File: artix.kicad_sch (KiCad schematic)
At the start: 50 parts, among them U2 XC7A200T-FBG484

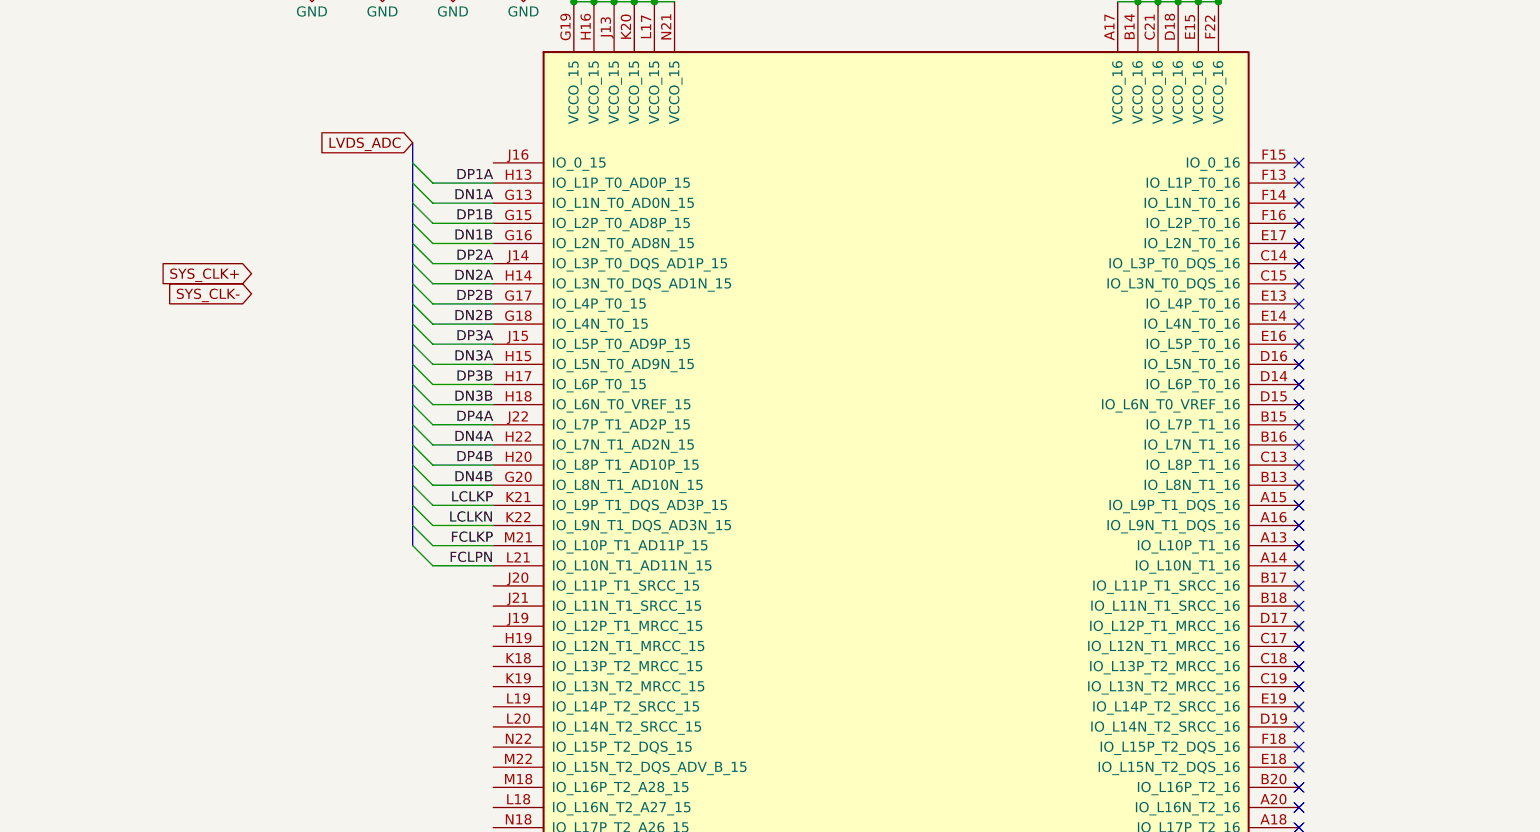
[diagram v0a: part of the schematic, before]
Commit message: added clk
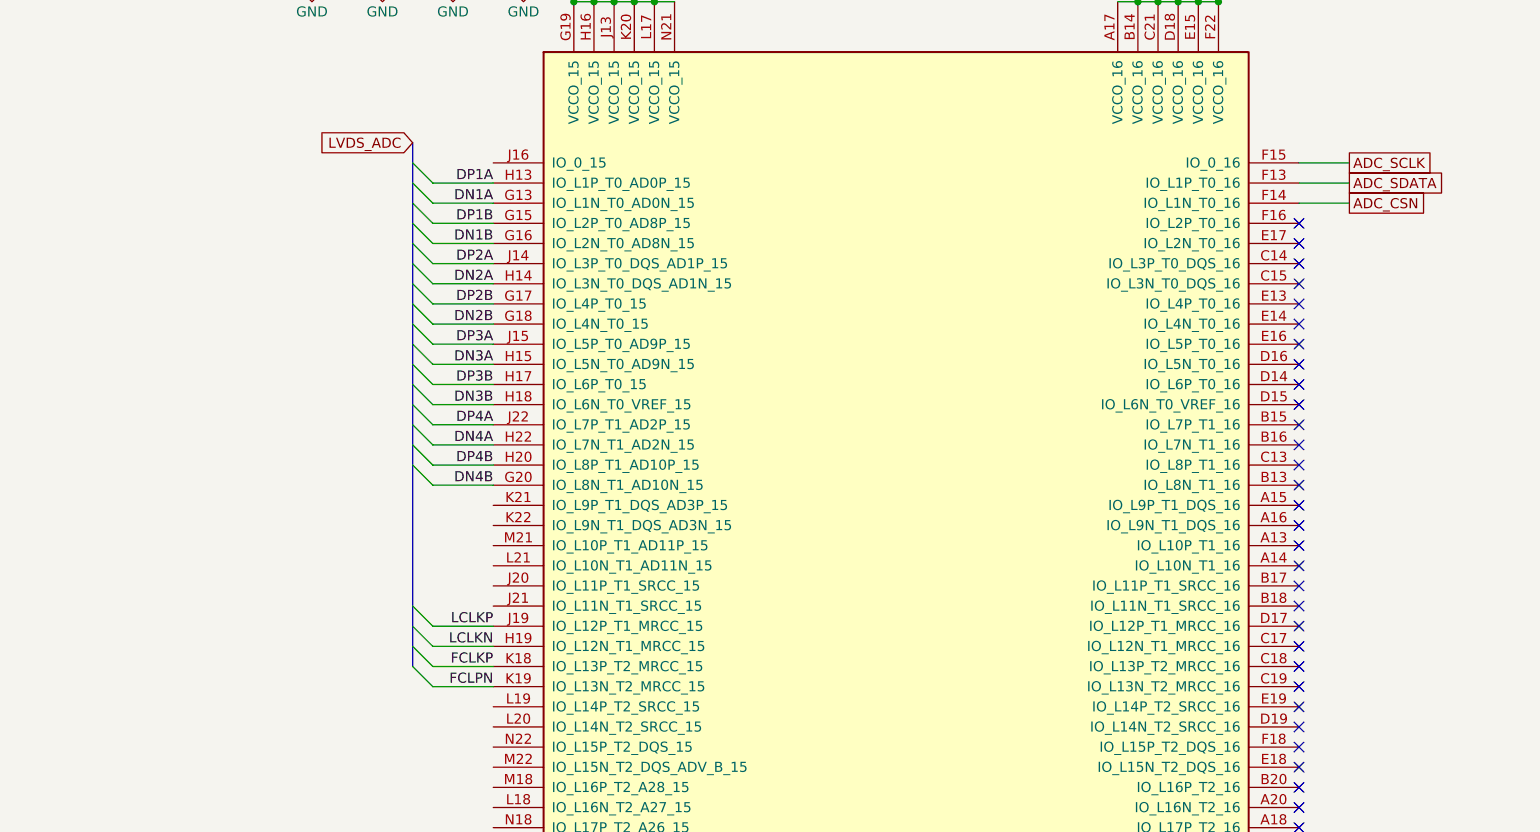
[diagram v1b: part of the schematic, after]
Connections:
- net FCLKP: now also U2.K18 (IO_L13P_T2_MRCC_15); no longer U2.M21 (IO_L10P_T1_AD11P_15)
- net FCLPN: now also U2.K19 (IO_L13N_T2_MRCC_15); no longer U2.L21 (IO_L10N_T1_AD11N_15)
- net LCLKN: now also U2.H19 (IO_L12N_T1_MRCC_15); no longer U2.K22 (IO_L9N_T1_DQS_AD3N_15)
- net LCLKP: now also U2.J19 (IO_L12P_T1_MRCC_15); no longer U2.K21 (IO_L9P_T1_DQS_AD3P_15)
- net ADC_SDATA: now reaches U2.F13 (IO_L1P_T0_16)
- net ADC_CSN: now reaches U2.F14 (IO_L1N_T0_16)
- net ADC_SCLK: now reaches U2.F15 (IO_0_16)
- no-connect marks 180 -> 177
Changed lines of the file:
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@@
 	)
 	(no_connect
-		(at 541.02 92.71)
-	)
-	(no_connect
 		(at 541.02 143.51)
 	)
 	(no_connect
-		(at 541.02 97.79)
-	)
-	(no_connect
 		(at 541.02 207.01)
 	)
@@
 	)
 	(no_connect
-		(at 541.02 95.25)
-	)
-	(no_connect
 		(at 140.97 176.53)
 	)
@@
 	)
 	(bus_entry
-		(at 431.8 95.25)
+		(at 431.8 158.75)
 		(size -2.54 -2.54)
 		(stroke
@@
 	)
 	(bus_entry
-		(at 431.8 135.89)
+		(at 431.8 95.25)
 		(size -2.54 -2.54)
 		(stroke
@@
 	)
 	(bus_entry
-		(at 431.8 110.49)
+		(at 431.8 153.67)
 		(size -2.54 -2.54)
 		(stroke
@@
 	)
 	(bus_entry
-		(at 431.8 128.27)
+		(at 431.8 110.49)
 		(size -2.54 -2.54)
 		(stroke
@@
 	)
 	(bus_entry
-		(at 431.8 140.97)
+		(at 431.8 128.27)
 		(size -2.54 -2.54)
 		(stroke
@@
 	)
 	(bus_entry
-		(at 431.8 143.51)
+		(at 431.8 151.13)
 		(size -2.54 -2.54)
 		(stroke
@@
 	)
 	(bus_entry
-		(at 431.8 138.43)
+		(at 431.8 105.41)
 		(size -2.54 -2.54)
 		(stroke
@@
 	)
 	(bus_entry
-		(at 431.8 105.41)
+		(at 431.8 156.21)
 		(size -2.54 -2.54)
 		(stroke
@@
 	(wire
 		(pts
-			(xy 439.42 138.43) (xy 431.8 138.43)
+			(xy 238.76 49.53) (xy 238.76 50.8)
 		)
 		(stroke
@@
 	(wire
 		(pts
-			(xy 238.76 49.53) (xy 238.76 50.8)
+			(xy 22.86 41.91) (xy 22.86 43.18)
 		)
 		(stroke
@@
 	(wire
 		(pts
-			(xy 22.86 41.91) (xy 22.86 43.18)
+			(xy 439.42 158.75) (xy 431.8 158.75)
 		)
 		(stroke
@@
 	(wire
 		(pts
+			(xy 541.02 97.79) (xy 547.37 97.79)
+		)
+		(stroke
+			(width 0)
+			(type default)
+		)
+	)
+	(wire
+		(pts
 			(xy 380.365 60.96) (xy 380.365 61.595)
 		)
@@
 	(wire
 		(pts
-			(xy 439.42 135.89) (xy 431.8 135.89)
+			(xy 273.05 293.37) (xy 284.48 293.37)
 		)
 		(stroke
@@
 	(wire
 		(pts
-			(xy 273.05 293.37) (xy 284.48 293.37)
+			(xy 541.02 95.25) (xy 547.37 95.25)
 		)
 		(stroke
@@
 	(bus
 		(pts
-			(xy 429.26 90.17) (xy 429.26 140.97)
+			(xy 429.26 90.17) (xy 429.26 156.21)
 		)
 		(stroke
@@
 	(wire
 		(pts
-			(xy 439.42 143.51) (xy 431.8 143.51)
+			(xy 541.02 92.71) (xy 547.37 92.71)
 		)
 		(stroke
@@
 	(wire
 		(pts
+			(xy 439.42 153.67) (xy 431.8 153.67)
+		)
+		(stroke
+			(width 0)
+			(type default)
+		)
+	)
+	(wire
+		(pts
 			(xy 439.42 105.41) (xy 431.8 105.41)
 		)
@@
 	(wire
 		(pts
+			(xy 439.42 156.21) (xy 431.8 156.21)
+		)
+		(stroke
+			(width 0)
+			(type default)
+		)
+	)
+	(wire
+		(pts
 			(xy 425.45 55.88) (xy 425.45 57.15)
 		)
@@
 	(wire
 		(pts
-			(xy 439.42 140.97) (xy 431.8 140.97)
-		)
-		(stroke
-			(width 0)
-			(type default)
-		)
-	)
-	(wire
-		(pts
 			(xy 146.05 48.26) (xy 146.05 48.895)
 		)
@@
 	(wire
 		(pts
+			(xy 439.42 151.13) (xy 431.8 151.13)
+		)
+		(stroke
+			(width 0)
+			(type default)
+		)
+	)
+	(wire
+		(pts
 			(xy 546.1 50.8) (xy 546.1 52.07)
 		)
@@
 		)
 	)
-	(label "DP4B"
-		(at 439.42 130.81 180)
+	(label "LCLKN"
+		(at 439.42 153.67 180)
 		(effects
 			(font
@@
 		)
 	)
-	(label "DP3B"
-		(at 439.42 120.65 180)
+	(label "FCLKP"
+		(at 439.42 156.21 180)
 		(effects
 			(font
@@
 		)
 	)
-	(label "FCLPN"
-		(at 439.42 143.51 180)
+	(label "DP4B"
+		(at 439.42 130.81 180)
+		(effects
+			(font
+				(size 1.27 1.27)
+			)
+			(justify right bottom)
+		)
+	)
+	(label "DP3B"
+		(at 439.42 120.65 180)
 		(effects
 			(font
@@
 		)
 	)
-	(label "FCLKP"
-		(at 439.42 140.97 180)
-		(effects
-			(font
-				(size 1.27 1.27)
-			)
-			(justify right bottom)
-		)
-	)
 	(label "DN3A"
 		(at 439.42 118.11 180)
@@
 		)
 	)
-	(label "DP3A"
-		(at 439.42 115.57 180)
+	(label "FCLPN"
+		(at 439.42 158.75 180)
 		(effects
 			(font
@@
 		)
 	)
-	(label "LCLKP"
-		(at 439.42 135.89 180)
+	(label "DP3A"
+		(at 439.42 115.57 180)
 		(effects
 			(font
@@
 		)
 	)
-	(label "LCLKN"
-		(at 439.42 138.43 180)
+	(label "DN2B"
+		(at 439.42 113.03 180)
 		(effects
 			(font
@@
 		)
 	)
-	(label "DN2B"
-		(at 439.42 113.03 180)
+	(label "LCLKP"
+		(at 439.42 151.13 180)
 		(effects
 			(font
@@
 		)
 	)
+	(global_label "ADC_SCLK"
+		(shape passive)
+		(at 547.37 92.71 0)
+		(effects
+			(font
+				(size 1.27 1.27)
+			)
+			(justify left)
+		)
+		(property "Intersheetrefs" "${INTERSHEET_REFS}"
+			(at 547.37 92.71 0)
+			(hide yes)
+			(show_name no)
+			(do_not_autoplace no)
+			(effects
+				(font
+					(size 1.27 1.27)
+				)
+			)
+		)
+	)
 	(global_label "QSPI_CS"
 		(shape input)
@@
 		)
 	)
+	(global_label "ADC_CSN"
+		(shape passive)
+		(at 547.37 97.79 0)
+		(effects
+			(font
+				(size 1.27 1.27)
+			)
+			(justify left)
+		)
+		(property "Intersheetrefs" "${INTERSHEET_REFS}"
+			(at 547.37 97.79 0)
+			(hide yes)
+			(show_name no)
+			(do_not_autoplace no)
+			(effects
+				(font
+					(size 1.27 1.27)
+				)
+			)
+		)
+	)
 	(global_label "MGTPRX2_216+"
 		(shape bidirectional)
@@
 		)
 	)
-	(global_label "SYS_CLK-"
-		(shape input)
-		(at 408.94 109.22 180)
-		(fields_autoplaced yes)
+	(global_label "ADC_SDATA"
+		(shape passive)
+		(at 547.37 95.25 0)
 		(effects
 			(font
 				(size 1.27 1.27)
 			)
-			(justify right)
+			(justify left)
 		)
 		(property "Intersheetrefs" "${INTERSHEET_REFS}"
-			(at 396.3391 109.22 0)
+			(at 547.37 95.25 0)
 			(hide yes)
 			(show_name no)
@@
 					(size 1.27 1.27)
 				)
-				(justify right)
 			)
 		)
@@
 			)
 		)
-	)
-	(global_label "SYS_CLK+"
-		(shape input)
-		(at 408.94 106.68 180)
-		(fields_autoplaced yes)
-		(effects
-			(font
-				(size 1.27 1.27)
-			)
-			(justify right)
-		)
-		(property "Intersheetrefs" "${INTERSHEET_REFS}"
-			(at 396.3391 106.68 0)
-			(hide yes)
-			(show_name no)
-			(do_not_autoplace no)
-			(effects
-				(font
-					(size 1.27 1.27)
-				)
-				(justify right)
-			)
-		)
